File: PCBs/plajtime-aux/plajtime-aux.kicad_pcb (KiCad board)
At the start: 2 copper layers, 50.7 x 23.5 mm, 21 parts, among them J1 Slider, J2 USB, J3 Internal connector, J4 LRA, U1 USBLC6-2P6, U2 IQS7222B, U3 DA7280

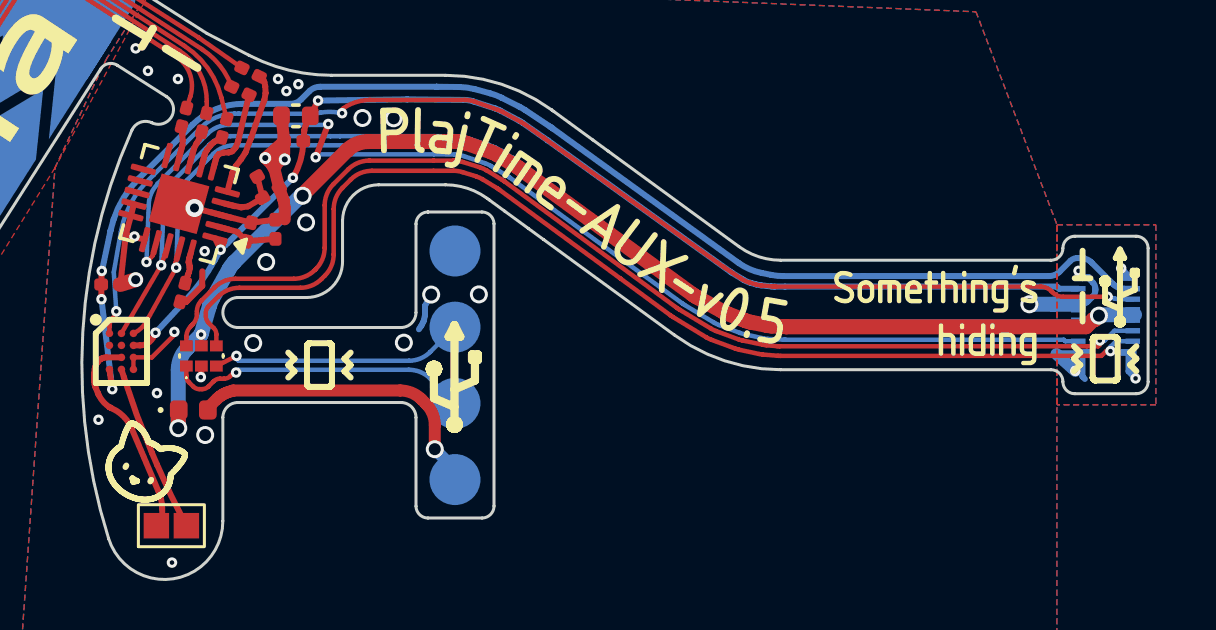
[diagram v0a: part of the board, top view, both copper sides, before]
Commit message: All production fixes
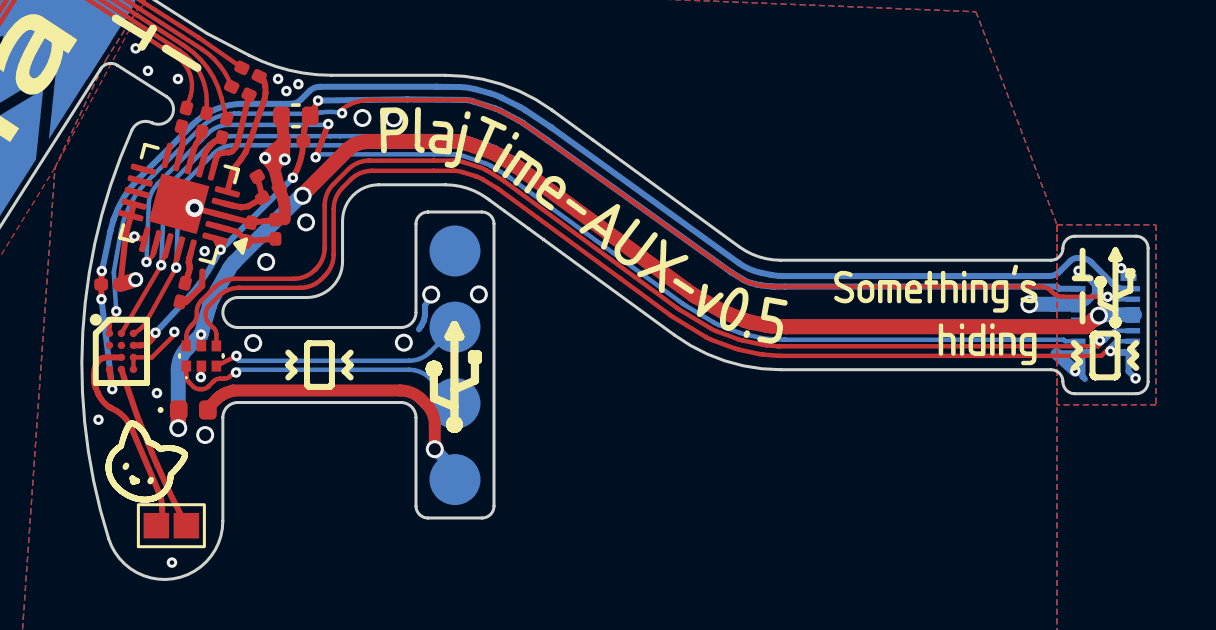
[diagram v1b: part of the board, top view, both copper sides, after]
